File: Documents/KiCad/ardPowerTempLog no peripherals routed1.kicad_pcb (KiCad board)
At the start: 2 copper layers, 26 parts, among them J10 5-pin_3-pole_3,5mm_audio_head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, J11 4-pin_3LED_header, J12 Conn_01x02_Male, J13 Conn_01x02_Male, J6 5-pin_3-pole_3,5mm_audio_head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, J7 5-pin_3-pole_3,5mm_audio_head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, J8 5-pin_3-pole_3,5mm_audio_head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, J9 5-pin_3-pole_3,5mm_audio_head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

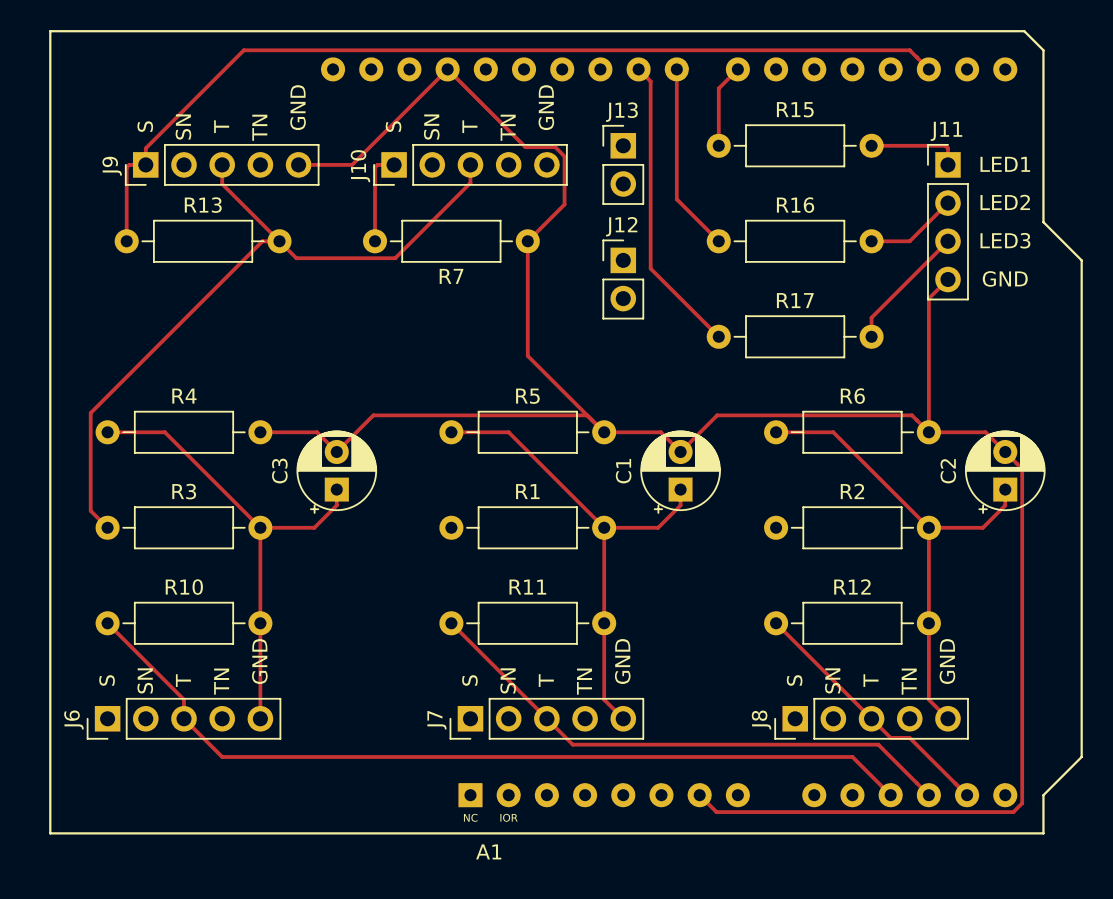
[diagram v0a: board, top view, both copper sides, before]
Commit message: schematics
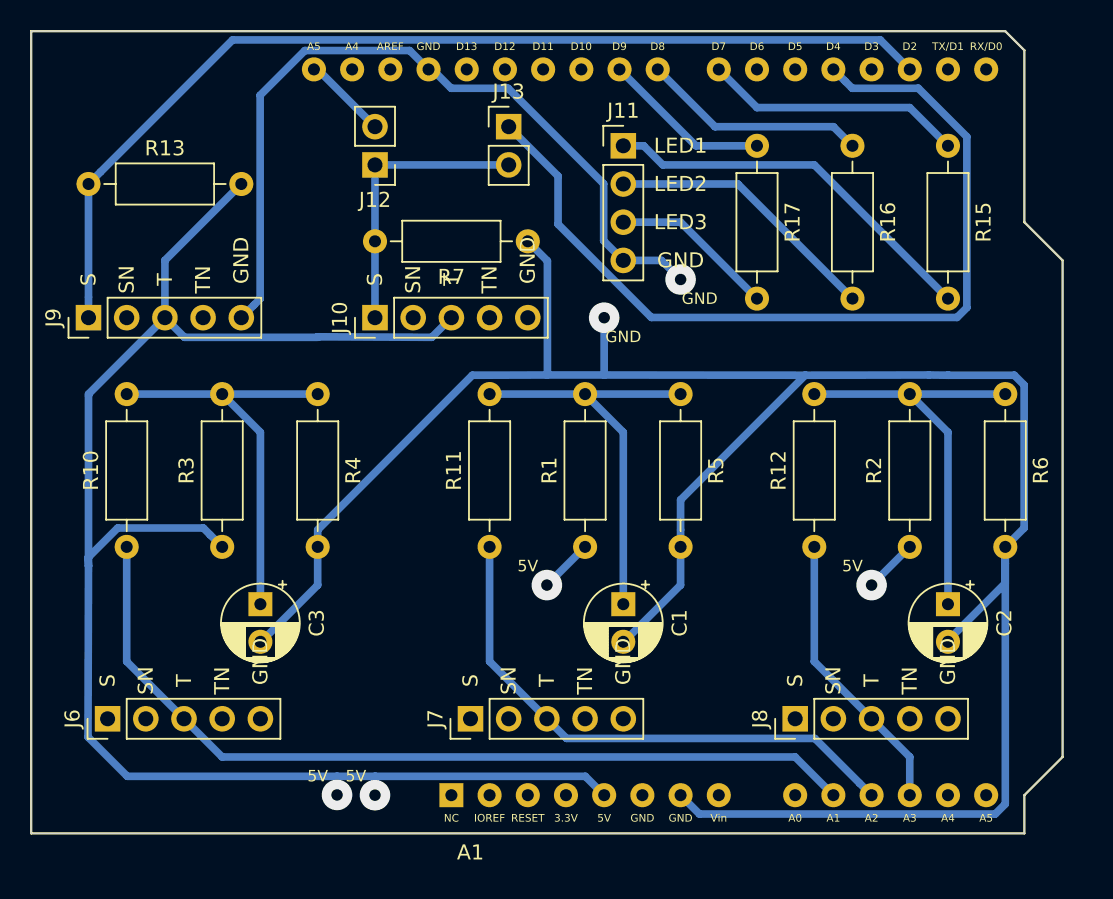
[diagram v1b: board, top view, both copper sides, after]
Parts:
- R6: value 100k -> 10k
- moved J11 21.6 mm to (144.8, 66.0)
- moved J12 17.7 mm to (128.3, 67.3), turned to 180 degrees
- moved R5 15.5 mm to (148.6, 82.5), turned to 270 degrees
- moved R6 15.5 mm to (170.2, 82.5), turned to 270 degrees
- moved R15 15.2 mm to (166.4, 66.0), turned to 270 degrees
- moved R4 14.2 mm to (124.5, 82.5), turned to 270 degrees
- moved R17 13.0 mm to (153.7, 66.0), turned to 270 degrees
- moved R16 10.9 mm to (160.0, 66.0), turned to 270 degrees
- moved J9 10.9 mm to (109.2, 77.5)
- moved J10 10.2 mm to (128.3, 77.5)
- moved C3 9.16 mm to (120.7, 96.5), turned to 270 degrees
- moved R1 8.98 mm to (142.2, 92.7), turned to 90 degrees
- moved R2 8.98 mm to (163.8, 92.7), turned to 90 degrees
- moved C1 8.52 mm to (144.8, 96.5), turned to 270 degrees
- moved C2 8.52 mm to (166.4, 96.5), turned to 270 degrees
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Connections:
- J12 pad 2: Net-(A1-Pad10) -> Net-(A1-Pad32)
- J6 pad 3: Net-(A1-Pad11) -> Net-(A1-Pad10)
- J7 pad 3: Net-(A1-Pad12) -> Net-(A1-Pad11)
- J8 pad 3: Net-(A1-Pad13) -> Net-(A1-Pad12)
- R10 pad 1: Net-(A1-Pad11) -> Net-(A1-Pad10)
- R11 pad 1: Net-(A1-Pad12) -> Net-(A1-Pad11)
- R12 pad 1: Net-(A1-Pad13) -> Net-(A1-Pad12)
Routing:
- net /Collector: track 48.5 -> 117.6 mm, vias 0 -> 4
- net Net-(A1-Pad19): track 0.00 -> 60.0 mm
- net Net-(A1-Pad10): track 0.00 -> 58.3 mm
- net /GND: track 154.9 -> 208.0 mm, vias 0 -> 2
- net Net-(A1-Pad11): track 57.5 -> 36.7 mm
- net Net-(D1-Pad2): track 6.25 -> 25.8 mm
- net Net-(A1-Pad13): track 18.6 -> 0.00 mm
- net Net-(A1-Pad12): track 36.5 -> 19.1 mm
- net /Emitter: track 6.25 -> 19.0 mm
- net Net-(D2-Pad2): track 6.13 -> 18.4 mm
- net Net-(A1-Pad22): track 5.61 -> 17.3 mm
- net Net-(A1-Pad24): track 20.0 -> 11.2 mm
- net /Data: track 62.6 -> 68.3 mm
- net Net-(A1-Pad32): track 0.00 -> 5.39 mm
- net Net-(C2-Pad1): track 32.8 -> 27.7 mm
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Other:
- board outline added: 68.6 x 53.3 mm
- board text added: "5V"
- board text added: "GND"
